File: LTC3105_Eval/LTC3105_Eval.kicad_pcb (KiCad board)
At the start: 2 copper layers, 29.1 x 15.2 mm, 14 parts, among them J1 Conn_01x05_Pin, J2 Conn_01x05_Pin, U1 LTC3105EMS

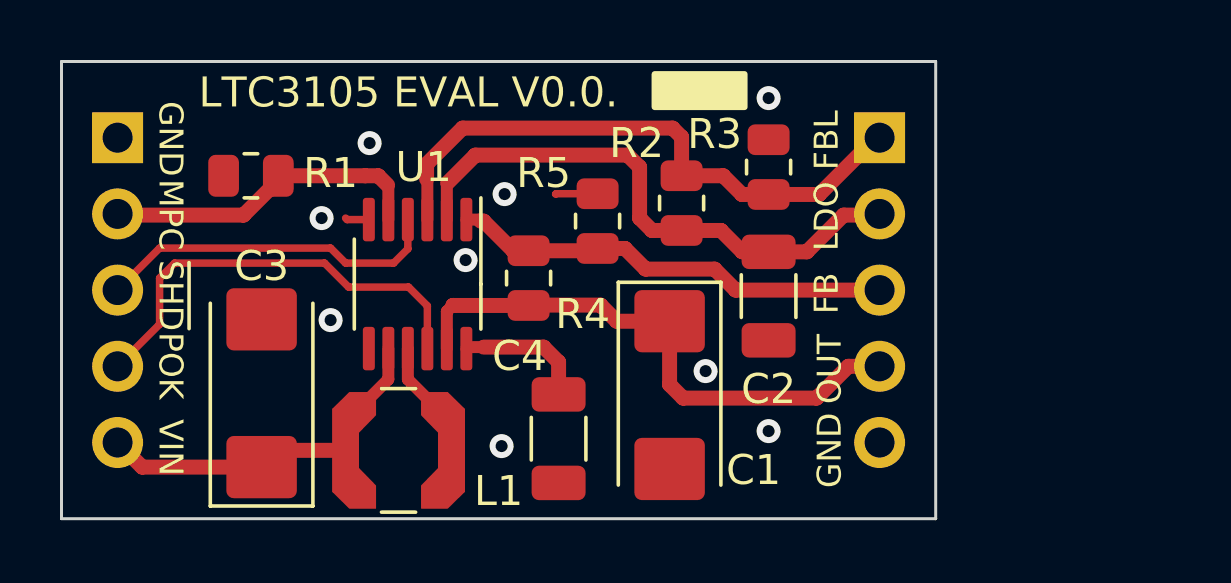
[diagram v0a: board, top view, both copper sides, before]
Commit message: work on issues
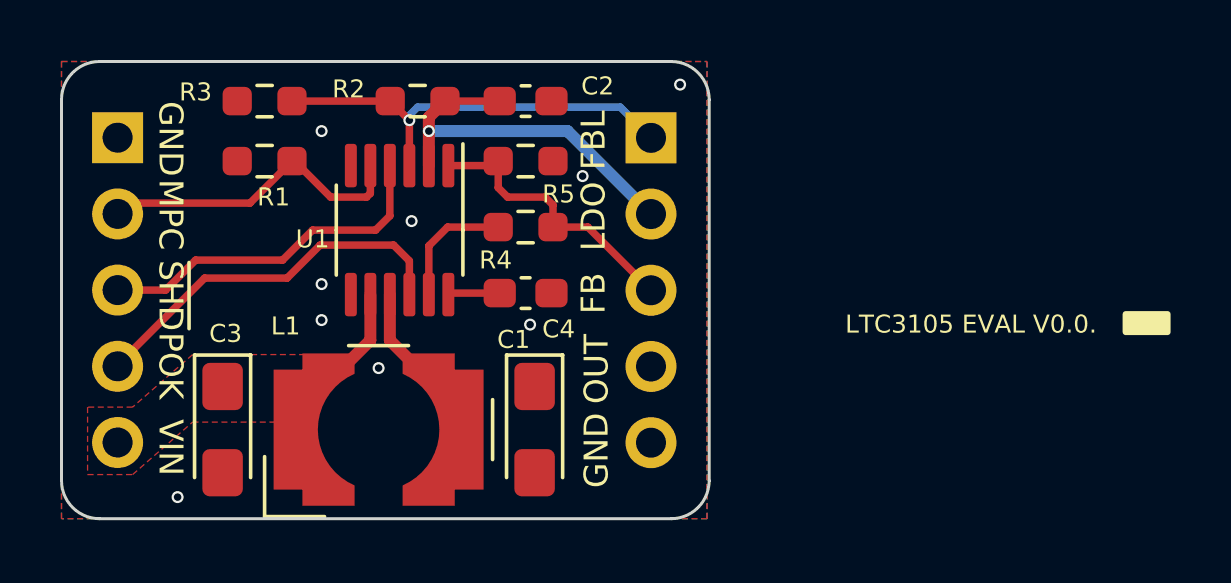
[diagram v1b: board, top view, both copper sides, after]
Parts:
- removed G***: LOGO, QRCODE.preety:LTC3105_Eval_V0_QRCode_5x5
- C1, C3: footprint Capacitor_Tantalum_SMD:CP_EIA-6032-28_Kemet-C -> Capacitor_Tantalum_SMD:CP_EIA-3216-18_Kemet-A_Pad1.58x1.35mm_HandSolder
- C2, C4: footprint Capacitor_SMD:C_1206_3216Metric -> Capacitor_SMD:C_0603_1608Metric_Pad1.08x0.95mm_HandSolder
- L1: value 10uF -> 10uH; footprint Inductor_SMD:L_Coilcraft_LPS4018 -> 021_inductor:L_Coilcraft_MSS5131-XXX_handsolder
- R1, R2, R3, R4, R5: footprint Resistor_SMD:R_0805_2012Metric -> Resistor_SMD:R_0603_1608Metric_Pad0.98x0.95mm_HandSolder
- moved R3 16.9 mm to (131.9, 95.3), turned to 180 degrees
- moved C2 10.4 mm to (140.6, 95.3), turned to 0 degrees
- moved R2 9.43 mm to (137.0, 95.3), turned to 180 degrees
- moved J2 7.62 mm to (144.8, 96.5)
- moved C4 4.98 mm to (140.6, 101.7), turned to 0 degrees
- moved C1 4.64 mm to (140.9, 106.2)
- moved R5 3.12 mm to (140.6, 97.3), turned to 0 degrees
- moved U1 1.90 mm to (136.4, 99.6)
- moved C3 1.78 mm to (130.5, 106.2), turned to -90 degrees
- moved R4 1.70 mm to (140.6, 99.5), turned to 0 degrees
- moved L1 0.96 mm to (135.7, 106.2), turned to 90 degrees
- moved R1 0.67 mm to (131.9, 97.3)
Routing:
- net VOUT: track 18.7 -> 4.20 mm
- net VIN: track 12.7 -> 2.55 mm
- net LDO_OUT: track 18.9 -> 12.7 mm, vias 0 -> 1
- net FB_LDO: track 19.9 -> 14.3 mm, vias 0 -> 1
- net FB: track 14.8 -> 9.55 mm
- net Net-(U1-AUX): track 4.38 -> 1.73 mm
- net GND: track 2.20 -> 0.00 mm
- net POWERGOOD: track 14.7 -> 12.8 mm
- net /SW: track 3.99 -> 2.69 mm
- added copper zone on F.Cu, net VIN
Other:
- board size 29.1 x 15.2 mm -> 21.6 x 15.2 mm
